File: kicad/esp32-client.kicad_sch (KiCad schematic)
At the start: 0 parts

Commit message: init
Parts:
- added U?: ESP32-C3-MINI-1, PCM_Espressif:ESP32-C3-MINI-1, symbol PCM_Espressif:ESP32-C3-MINI-1
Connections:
- new net: U?.1 (GND), U?.11 (GND), U?.14 (GND), U?.2 (GND), U?.36 (GND), U?.37 (GND), U?.38 (GND), U?.39 (GND), U?.40 (GND), U?.41 (GND), U?.42 (GND), U?.43 (GND), U?.44 (GND), U?.45 (GND), U?.46 (GND), U?.47 (GND), U?.48 (GND), U?.49 (GND), U?.50 (GND), U?.51 (GND), U?.52 (GND), U?.53 (GND)
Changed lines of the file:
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@@
 	(generator_version "9.0")
 	(paper "A4")
+	(symbol
+		(lib_id "PCM_Espressif:ESP32-C3-MINI-1")
+		(at 127 78.74 0)
+		(unit 1)
+		(exclude_from_sim no)
+		(in_bom yes)
+		(on_board yes)
+		(dnp no)
+		(fields_autoplaced yes)
+		(property "Reference" "U?"
+			(at 129.1433 48.26 0)
+			(effects
+				(font
+					(size 1.27 1.27)
+				)
+				(justify left)
+			)
+		)
+		(property "Value" "ESP32-C3-MINI-1"
+			(at 129.1433 50.8 0)
+			(effects
+				(font
+					(size 1.27 1.27)
+				)
+				(justify left)
+			)
+		)
+		(property "Footprint" "PCM_Espressif:ESP32-C3-MINI-1"
+			(at 127 114.3 0)
+			(effects
+				(font
+					(size 1.27 1.27)
+				)
+				(hide yes)
+			)
+		)
+		(property "Datasheet" "https://www.espressif.com/sites/default/files/documentation/esp32-c3-mini-1_datasheet_en.pdf"
+			(at 127 116.84 0)
+			(effects
+				(font
+					(size 1.27 1.27)
+				)
+				(hide yes)
+			)
+		)
+		(property "Description" "ESP32-C3-MINI-1 family is an ultra-low-power MCU-based SoC solution that supports 2.4 GHz Wi-Fi and Bluetooth®Low Energy (Bluetooth LE)."
+			(at 127 78.74 0)
+			(effects
+				(font
+					(size 1.27 1.27)
+				)
+				(hide yes)
+			)
+		)
+		(pin "15"
+		)
+		(pin "43"
+		)
+		(pin "6"
+		)
+		(pin "10"
+		)
+		(pin "32"
+		)
+		(pin "46"
+		)
+		(pin "50"
+		)
+		(pin "42"
+		)
+		(pin "39"
+		)
+		(pin "45"
+		)
+		(pin "19"
+		)
+		(pin "49"
+		)
+		(pin "17"
+		)
+		(pin "29"
+		)
+		(pin "14"
+		)
+		(pin "31"
+		)
+		(pin "44"
+		)
+		(pin "20"
+		)
+		(pin "52"
+		)
+		(pin "2"
+		)
+		(pin "21"
+		)
+		(pin "24"
+		)
+		(pin "5"
+		)
+		(pin "53"
+		)
+		(pin "51"
+		)
+		(pin "34"
+		)
+		(pin "48"
+		)
+		(pin "11"
+		)
+		(pin "36"
+		)
+		(pin "26"
+		)
+		(pin "30"
+		)
+		(pin "27"
+		)
+		(pin "16"
+		)
+		(pin "23"
+		)
+		(pin "37"
+		)
+		(pin "9"
+		)
+		(pin "7"
+		)
+		(pin "4"
+		)
+		(pin "13"
+		)
+		(pin "12"
+		)
+		(pin "28"
+		)
+		(pin "8"
+		)
+		(pin "18"
+		)
+		(pin "22"
+		)
+		(pin "38"
+		)
+		(pin "35"
+		)
+		(pin "3"
+		)
+		(pin "25"
+		)
+		(pin "40"
+		)
+		(pin "47"
+		)
+		(pin "33"
+		)
+		(pin "1"
+		)
+		(pin "41"
+		)
+		(instances
+			(project ""
+				(path "/4a001952-2620-48e5-963e-8cfcd99c6e64"
+					(reference "U?")
+					(unit 1)
+				)
+			)
+		)
+	)
 	(sheet_instances
 		(path "/"

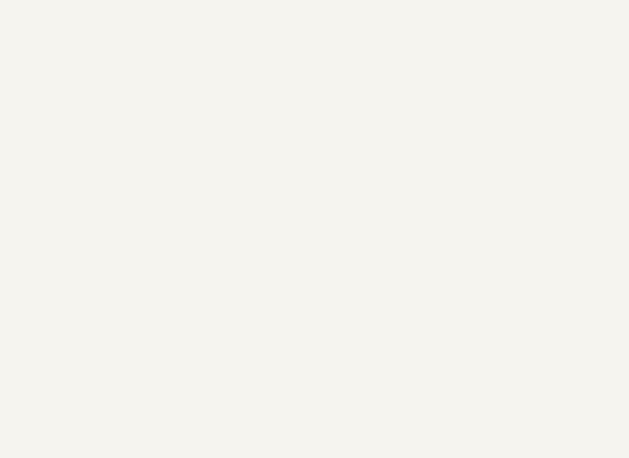
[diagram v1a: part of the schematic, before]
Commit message: init
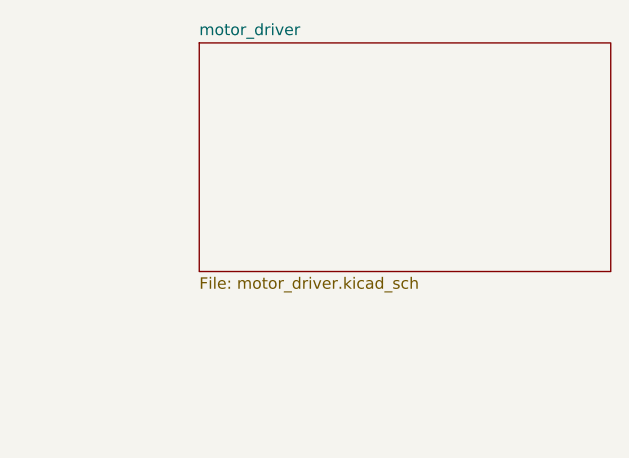
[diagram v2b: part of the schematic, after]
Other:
- added sheet motor_driver (motor_driver.kicad_sch)
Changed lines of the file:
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@@
+		)
+	)
+	(sheet
+		(at 193.04 31.75)
+		(size 45.72 25.4)
+		(exclude_from_sim no)
+		(in_bom yes)
+		(on_board yes)
+		(dnp no)
+		(fields_autoplaced yes)
+		(stroke
+			(width 0.1524)
+			(type solid)
+		)
+		(fill
+			(color 0 0 0 0.0000)
+		)
+		(property "Sheetname" "motor_driver"
+			(at 193.04 31.0384 0)
+			(effects
+				(font
+					(size 1.27 1.27)
+				)
+				(justify left bottom)
+			)
+		)
+		(property "Sheetfile" "motor_driver.kicad_sch"
+			(at 193.04 57.7346 0)
+			(effects
+				(font
+					(size 1.27 1.27)
+				)
+				(justify left top)
+			)
+		)
+		(instances
+			(project "esp32-client"
+				(path "/4a001952-2620-48e5-963e-8cfcd99c6e64"
+					(page "2")
+				)
+			)
 		)
 	)
